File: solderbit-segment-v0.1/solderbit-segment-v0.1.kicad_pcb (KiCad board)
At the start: 2 copper layers, 25 x 50 mm, 15 parts, among them J1 Conn_01x05_Pin, U1 PCF8574AT, U2 PCF8574N

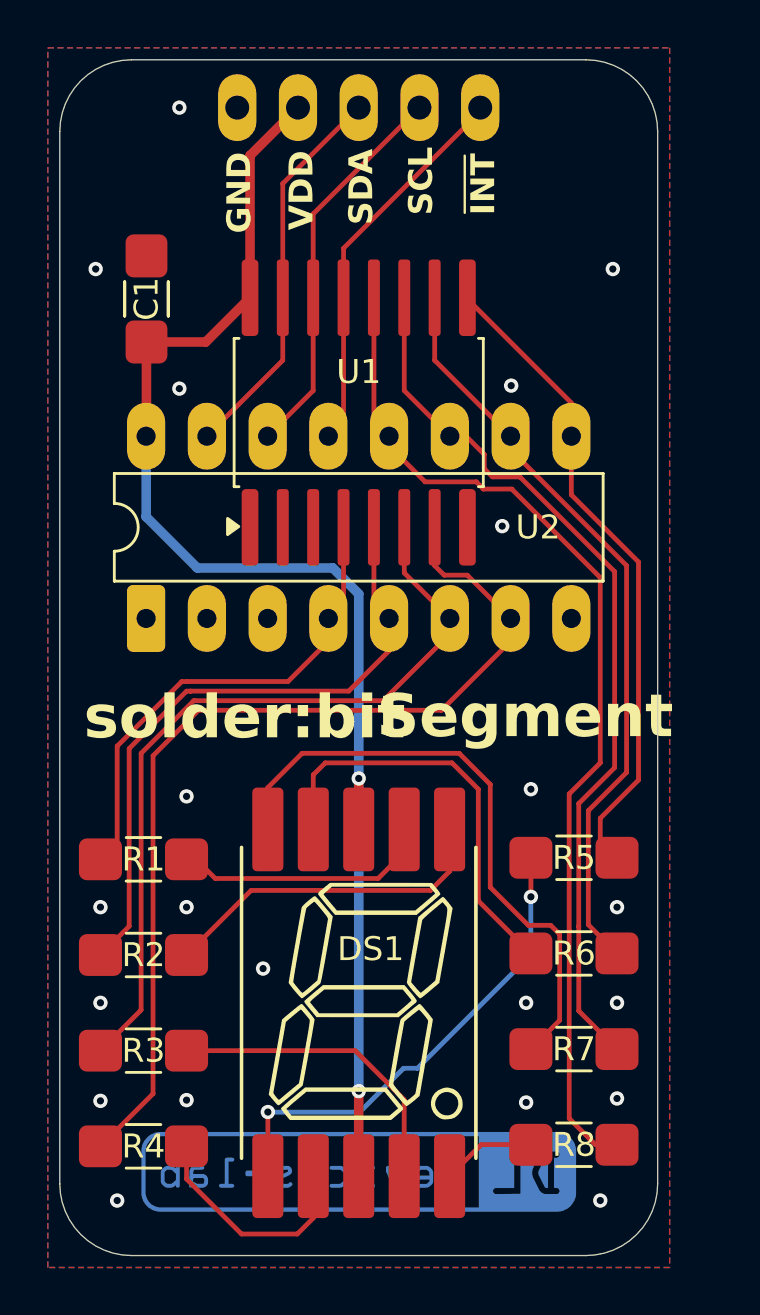
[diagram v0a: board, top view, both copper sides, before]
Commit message: New documentation
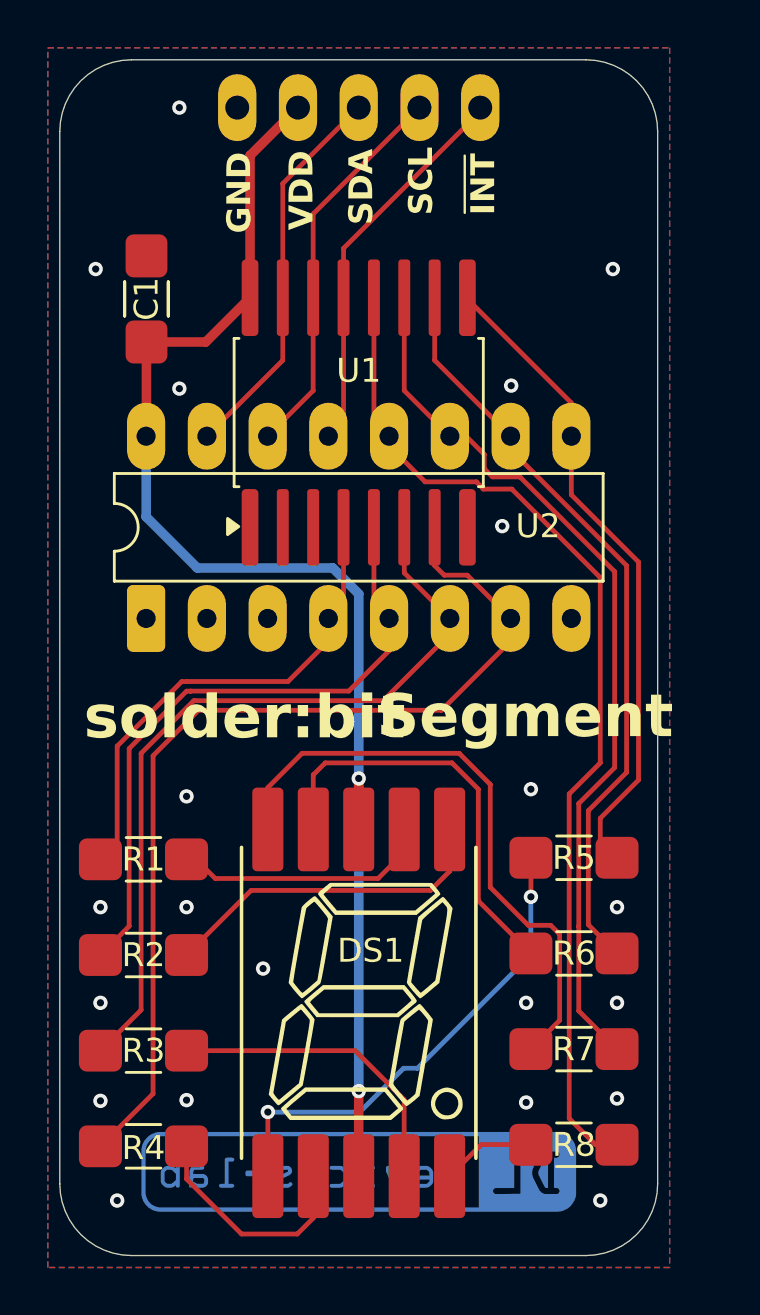
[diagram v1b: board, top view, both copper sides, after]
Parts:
- C1: footprint SolderbitSegment:C_1206 -> Solderbit_Segment:C_1206
- DS1: footprint SolderbitSegment:VDMR10 -> Solderbit_Segment:VDMR10
- J1: footprint SolderbitSegment:PinHeader_1x05_P2.54mm_Vertical -> Solderbit_Segment:PinHeader_1x05_P2.54mm_Vertical
- R1, R2, R3, R4, R5, R6, R7, R8: footprint SolderbitSegment:R_1206 -> Solderbit_Segment:R_1206
- U1: footprint SolderbitSegment:SO-16 -> Solderbit_Segment:SO-16
- U2: footprint SolderbitSegment:DIP-16 -> Solderbit_Segment:DIP-16
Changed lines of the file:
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@@
 	(net 20 "Net-(DS1-G)")
 	(net 21 "Net-(DS1-E)")
-	(footprint "SolderbitSegment:R_1206"
+	(footprint "Solderbit_Segment:R_1206"
 		(layer "F.Cu")
 		(at 149 90.3675 180)
@@
 		(tags "resistor handsolder")
 		(property "Reference" "R5"
-			(at 0 0 0)
+			(at 0 0 180)
 			(layer "F.SilkS")
 			(effects
@@
 		)
 		(property "Value" "150R"
-			(at 0 1.83 0)
+			(at 0 1.83 180)
 			(layer "F.Fab")
 			(hide yes)
@@
 		)
 		(property "Datasheet" "https://yageogroup.com/content/datasheet/asset/file/PYU-RC_GROUP_51_ROHS_L"
-			(at 0 0 0)
+			(at 0 0 180)
 			(layer "F.Fab")
 			(hide yes)
@@
 		)
 		(property "Description" "Resistor, small US symbol"
-			(at 0 0 0)
+			(at 0 0 180)
 			(layer "F.Fab")
 			(hide yes)
@@
 		)
 		(fp_text user "${REFERENCE}"
-			(at 0 0 0)
+			(at 0 0 180)
 			(layer "F.Fab")
 			(effects
@@
 		)
 	)
-	(footprint "SolderbitSegment:R_1206"
+	(footprint "Solderbit_Segment:R_1206"
 		(layer "F.Cu")
 		(at 131 94.4325)
@@
 		)
 	)
-	(footprint "SolderbitSegment:R_1206"
+	(footprint "Solderbit_Segment:R_1206"
 		(layer "F.Cu")
 		(at 149 94.3675 180)
@@
 		(tags "resistor handsolder")
 		(property "Reference" "R6"
-			(at 0 0 0)
+			(at 0 0 180)
 			(layer "F.SilkS")
 			(effects
@@
 		)
 		(property "Value" "150R"
-			(at 0 1.83 0)
+			(at 0 1.83 180)
 			(layer "F.Fab")
 			(hide yes)
@@
 		)
 		(property "Datasheet" "https://yageogroup.com/content/datasheet/asset/file/PYU-RC_GROUP_51_ROHS_L"
-			(at 0 0 0)
+			(at 0 0 180)
 			(layer "F.Fab")
 			(hide yes)
@@
 		)
 		(property "Description" "Resistor, small US symbol"
-			(at 0 0 0)
+			(at 0 0 180)
 			(layer "F.Fab")
 			(hide yes)
@@
 		)
 		(fp_text user "${REFERENCE}"
-			(at 0 0 0)
+			(at 0 0 180)
 			(layer "F.Fab")
 			(effects
@@
 		)
 	)
-	(footprint "SolderbitSegment:R_1206"
+	(footprint "Solderbit_Segment:R_1206"
 		(layer "F.Cu")
 		(at 131 90.4325)
@@
 		)
 	)
-	(footprint "SolderbitSegment:VDMR10"
+	(footprint "Solderbit_Segment:VDMR10"
 		(layer "F.Cu")
 		(at 140 96.4325)
 		(property "Reference" "DS1"
-			(at 0.5 -2.25 0)
+			(at 0.5 -2.1825 0)
 			(unlocked yes)
 			(layer "F.SilkS")
@@
 		)
 		(property "Value" "VDMO10A0"
-			(at 0 -16.3 0)
+			(at 0 -11.3 0)
 			(unlocked yes)
 			(layer "F.Fab")
-			(hide yes)
 			(effects
 				(font
@@
 		)
 		(group ""
-			(members "06b99de5-cb5e-4bf8-9ea6-f26118e50e92" "2b57747c-4ed4-4840-b80f-a78707ac252b"
-				"32e729c5-9c12-45be-9830-76d494841fcf" "6277aeaa-1453-4d52-a125-25ed458209b9"
-				"c132c745-aa8b-4a8b-a377-c740b8591b62" "e916a083-963e-4db6-8546-0362b82ae70d"
-				"f854aeb2-3b0d-4c3e-9791-75dd08fc1365" "ff2eabd7-3149-4cad-abe6-33c12c2fd23c"
+			(members "085b431f-c60e-4b92-8bce-c3aa19fc89ac" "4027ebb5-f6d5-46b6-8540-c3a557c738f9"
+				"4f03b84b-5639-4d59-a86d-37a38fe639dd" "78b857af-609a-4701-9978-d15a27971585"
+				"c11c2262-25d2-4b71-9e59-c0299c79da08" "c19a8c33-9f4a-4a81-bdc4-4a93684ac2ab"
+				"cf1362d4-c866-46b8-94de-2c6f71d6ec74" "f63f0a59-3310-4aa9-9875-b032bf7d925a"
 			)
 		)
 		(embedded_fonts no)
-		(model "${KIPRJMOD}/library/SolderbitSegment.3dshapes/VDMR10A0.stp"
+		(model "${KIPRJMOD}/library/Solderbit_Segment.3dshapes/VDMR10A0.stp"
 			(offset
 				(xyz 0 0 0)
@@
 		)
 	)
-	(footprint "SolderbitSegment:R_1206"
+	(footprint "Solderbit_Segment:R_1206"
 		(layer "F.Cu")
 		(at 131 98.4325)
@@
 		)
 	)
-	(footprint "SolderbitSegment:C_1206"
+	(footprint "Solderbit_Segment:C_1206"
 		(layer "F.Cu")
 		(at 131.125 67 90)
@@
 			(at 0 1.85 90)
 			(layer "F.Fab")
-			(hide yes)
 			(effects
 				(font
@@
 		)
 	)
-	(footprint "SolderbitSegment:R_1206"
+	(footprint "Solderbit_Segment:R_1206"
 		(layer "F.Cu")
 		(at 149 98.3675 180)
@@
 		(tags "resistor handsolder")
 		(property "Reference" "R7"
-			(at 0 0 0)
+			(at 0 0 180)
 			(layer "F.SilkS")
 			(effects
@@
 		)
 		(property "Value" "150R"
-			(at 0 1.83 0)
+			(at 0 1.83 180)
 			(layer "F.Fab")
 			(hide yes)
@@
 		)
 		(property "Datasheet" "https://yageogroup.com/content/datasheet/asset/file/PYU-RC_GROUP_51_ROHS_L"
-			(at 0 0 0)
+			(at 0 0 180)
 			(layer "F.Fab")
 			(hide yes)
@@
 		)
 		(property "Description" "Resistor, small US symbol"
-			(at 0 0 0)
+			(at 0 0 180)
 			(layer "F.Fab")
 			(hide yes)
@@
 		)
 		(fp_text user "${REFERENCE}"
-			(at 0 0 0)
+			(at 0 0 180)
 			(layer "F.Fab")
 			(effects
@@
 		)
 	)
-	(footprint "SolderbitSegment:SO-16"
+	(footprint "Solderbit_Segment:SO-16"
 		(layer "F.Cu")
 		(at 140 71.75 90)
@@
 		(tags "SO SO")
 		(property "Reference" "U1"
-			(at 1.7 0 180)
+			(at 1.75 0 180)
 			(layer "F.SilkS")
 			(effects
@@
 			(at 0 6.05 90)
 			(layer "F.Fab")
-			(hide yes)
 			(effects
 				(font
@@
 		(sheetname "/")
 		(sheetfile "solderbit-segment.kicad_sch")
-		(attr smd allow_missing_courtyard dnp)
+		(attr smd dnp)
 		(fp_line
 			(start 3.1 -5.21)
@@
 		)
 		(fp_text user "${REFERENCE}"
-			(at 0 0 90)
+			(at 0 0 180)
 			(layer "F.Fab")
 			(effects
@@
 		)
 		(embedded_fonts no)
-		(model "${KIPRJMOD}/library/SolderbitSegment.3dshapes/PCF8574AT_3,518.stp"
-			(hide yes)
+		(model "${KIPRJMOD}/library/Solderbit_Segment.3dshapes/PCF8574AT_3,518.stp"
 			(offset
 				(xyz 0 0 0)
@@
 		)
 	)
-	(footprint "SolderbitSegment:R_1206"
+	(footprint "Solderbit_Segment:R_1206"
 		(layer "F.Cu")
 		(at 131 102.4325)
@@
 		(tags "resistor handsolder")
 		(property "Reference" "R4"
-			(at 0 0 0)
+			(at 0 0.0675 0)
 			(layer "F.SilkS")
 			(effects
@@
 		)
 	)
-	(footprint "SolderbitSegment:R_1206"
+	(footprint "Solderbit_Segment:R_1206"
 		(layer "F.Cu")
 		(at 149 102.3675 180)
@@
 		(tags "resistor handsolder")
 		(property "Reference" "R8"
-			(at 0 0 0)
+			(at 0 0 180)
 			(layer "F.SilkS")
 			(effects
@@
 		)
 		(property "Value" "150R"
-			(at 0 1.83 0)
+			(at 0 1.83 180)
 			(layer "F.Fab")
 			(hide yes)
@@
 		)
 		(property "Datasheet" "https://yageogroup.com/content/datasheet/asset/file/PYU-RC_GROUP_51_ROHS_L"
-			(at 0 0 0)
+			(at 0 0 180)
 			(layer "F.Fab")
 			(hide yes)
@@
 		)
 		(property "Description" "Resistor, small US symbol"
-			(at 0 0 0)
+			(at 0 0 180)
 			(layer "F.Fab")
 			(hide yes)
@@
 		)
 		(fp_text user "${REFERENCE}"
-			(at 0 0 0)
+			(at 0 0 180)
 			(layer "F.Fab")
 			(effects
@@
 		)
 	)
-	(footprint "SolderbitSegment:DIP-16"
+	(footprint "Solderbit_Segment:DIP-16"
 		(layer "F.Cu")
 		(at 131.11 80.36 90)
@@
 		(tags "THT DIP DIL PDIP 2.54mm 7.62mm 300mil LongPads")
 		(property "Reference" "U2"
-			(at 3.81 16.39 180)
+			(at 3.86 16.39 180)
 			(layer "F.SilkS")
 			(effects
@@
 		(sheetname "/")
 		(sheetfile "solderbit-segment.kicad_sch")
-		(attr through_hole allow_missing_courtyard)
+		(attr through_hole)
 		(fp_line
 			(start 6.06 -1.33)
@@
 		)
 		(fp_text user "${REFERENCE}"
-			(at 3.81 8.89 0)
+			(at 3.81 8.89 180)
 			(layer "F.Fab")
 			(effects
@@
 		(embedded_fonts no)
 	)
-	(footprint "SolderbitSegment:PinHeader_1x05_P2.54mm_Vertical"
+	(footprint "Solderbit_Segment:PinHeader_1x05_P2.54mm_Vertical"
 		(layer "B.Cu")
 		(at 145.08 59 90)
@@
 		(tags "Through hole pin header THT 1x05 2.54mm single row")
 		(property "Reference" "J1"
-			(at 0 2.92 0)
+			(at 0 2.38 270)
 			(layer "B.SilkS")
 			(hide yes)
@@
 		)
 		(property "Value" "Conn_01x05_Pin"
-			(at 3 -5.08 0)
+			(at 0 -12.54 270)
 			(layer "B.Fab")
 			(hide yes)
@@
 		)
 		(property "Datasheet" "https://www.farnell.com/datasheets/1518407.pdf"
-			(at 0 0 90)
+			(at 0 0 270)
 			(layer "B.Fab")
 			(hide yes)
@@
 		)
 		(property "Description" "Generic connector, single row, 01x05, script generated"
-			(at 0 0 90)
+			(at 0 0 270)
 			(layer "B.Fab")
 			(hide yes)
@@
 		)
 		(fp_text user "${REFERENCE}"
-			(at 0 -5.08 0)
+			(at 0 -5.08 180)
 			(layer "B.Fab")
 			(effects
@@
 	)
 	(group ""
-		(members "104258c3-747b-4ba4-930f-86a382bfc2ca" "13c4efa7-a0e8-4ded-820f-3d01f7f30fc4"
-			"a640ebf3-b91e-4d9e-8d73-49922b609c5a" "e7cffdf9-6854-4e7d-9f12-206cccc8c29d"
-			"e8f8702f-edf8-4b0c-b553-2b335e70ed09"
-		)
-	)
-	(group ""
 		(members "06acc528-793c-4c2b-8d1d-cc87c42acc72" "4da83ed4-7bbf-4560-93eb-ed53cb029b0f"
 			"5af277a3-6f85-4fe2-b9fb-cb7b0d8ae642" "a16e1a46-512c-4f98-b465-a276b6d8ac15"
@@
 		)
 	)
+	(group ""
+		(members "13c4efa7-a0e8-4ded-820f-3d01f7f30fc4" "a640ebf3-b91e-4d9e-8d73-49922b609c5a"
+			"e7cffdf9-6854-4e7d-9f12-206cccc8c29d" "e8f8702f-edf8-4b0c-b553-2b335e70ed09"
+		)
+	)
